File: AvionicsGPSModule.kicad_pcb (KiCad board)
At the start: 4 copper layers, 60 x 56.1 mm, 34 parts, among them P1 MC311D, Q1 AO3400A, U1 RP2040, U2 AP2112K-3.3, U3 L80-R, U4 W25Q128JVS, X1 ABM8-272-T3

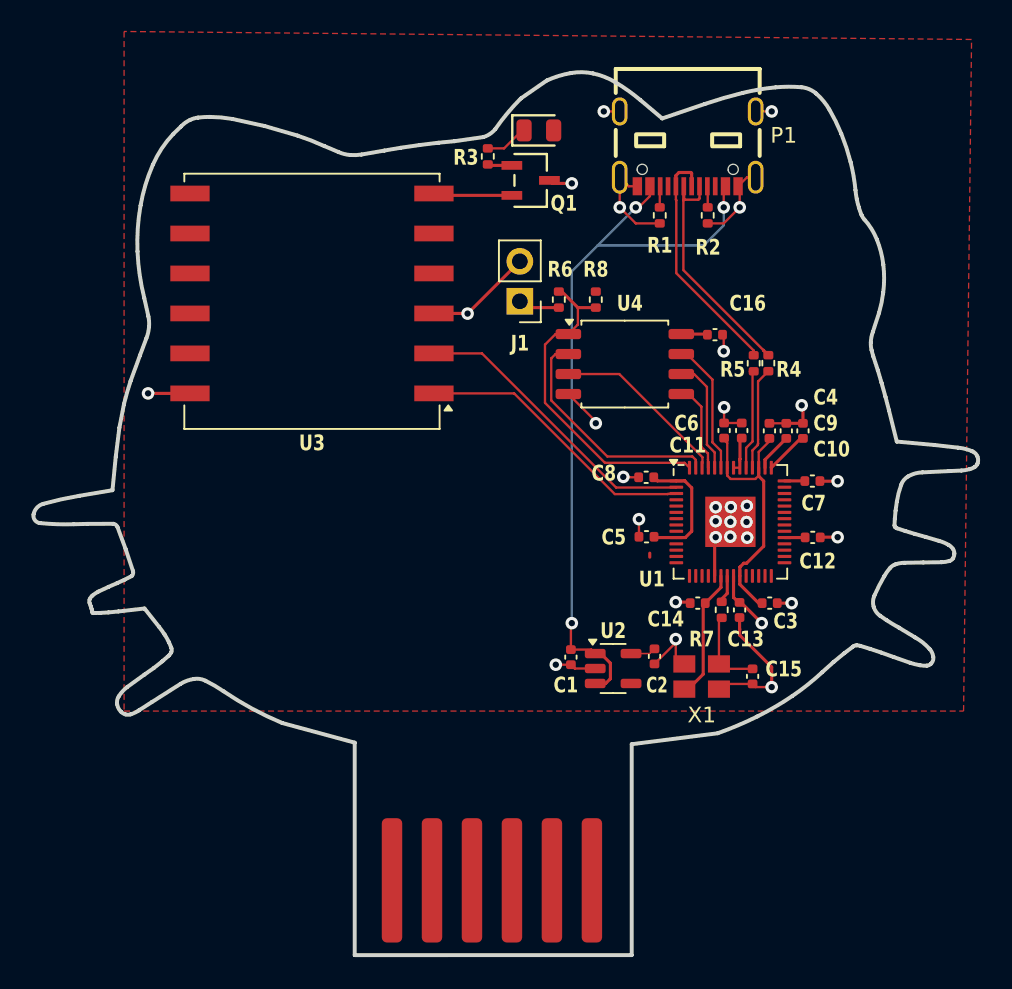
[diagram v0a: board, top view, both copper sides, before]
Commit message: minor changes
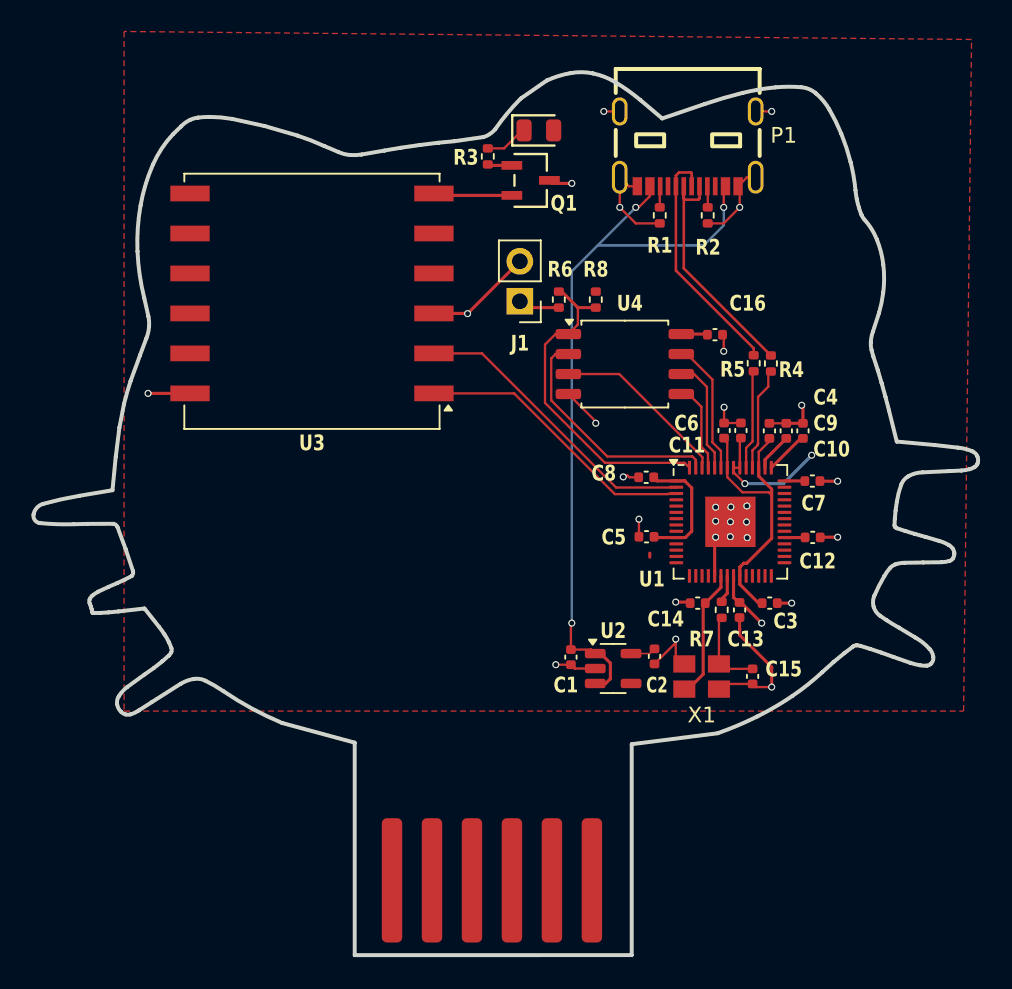
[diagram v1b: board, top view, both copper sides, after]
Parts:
- moved R4 0.17 mm to (153.9, 88.7)
- moved C11 0.05 mm to (152.0, 92.9)
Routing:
- net +3.3V: track 25.2 -> 31.9 mm, vias 1 -> 3
- net +1V1: track 17.5 -> 18.7 mm
